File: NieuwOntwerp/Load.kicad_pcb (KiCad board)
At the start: 2 copper layers, 84 x 96 mm, 151 parts, among them J1 USB_C_Receptacle_USB2.0, J10 Conn_01x02, J2 Conn_01x02, J3 Conn_01x03, J4 Conn_01x02, J5 Conn_01x09_Male, J6 Conn_01x02, J7 Conn_01x03, J8 Conn_01x02, J9 Conn_01x02, Q1 Si2306, Q2 4809NG, Q3 IRF840, Q4 IRF840, Q5 IRF840, Q6 Si2306, T1 EE13, U1 ESP12E, U10 PC817, U11 TL431, U12 LM1117-3.3, U2 FT231XQ, U3 LM358, U4 MCP4725A0, U5 LM358, U6 INA219, U7 PCF8574, U8 SSD1306, U9 LNK364D

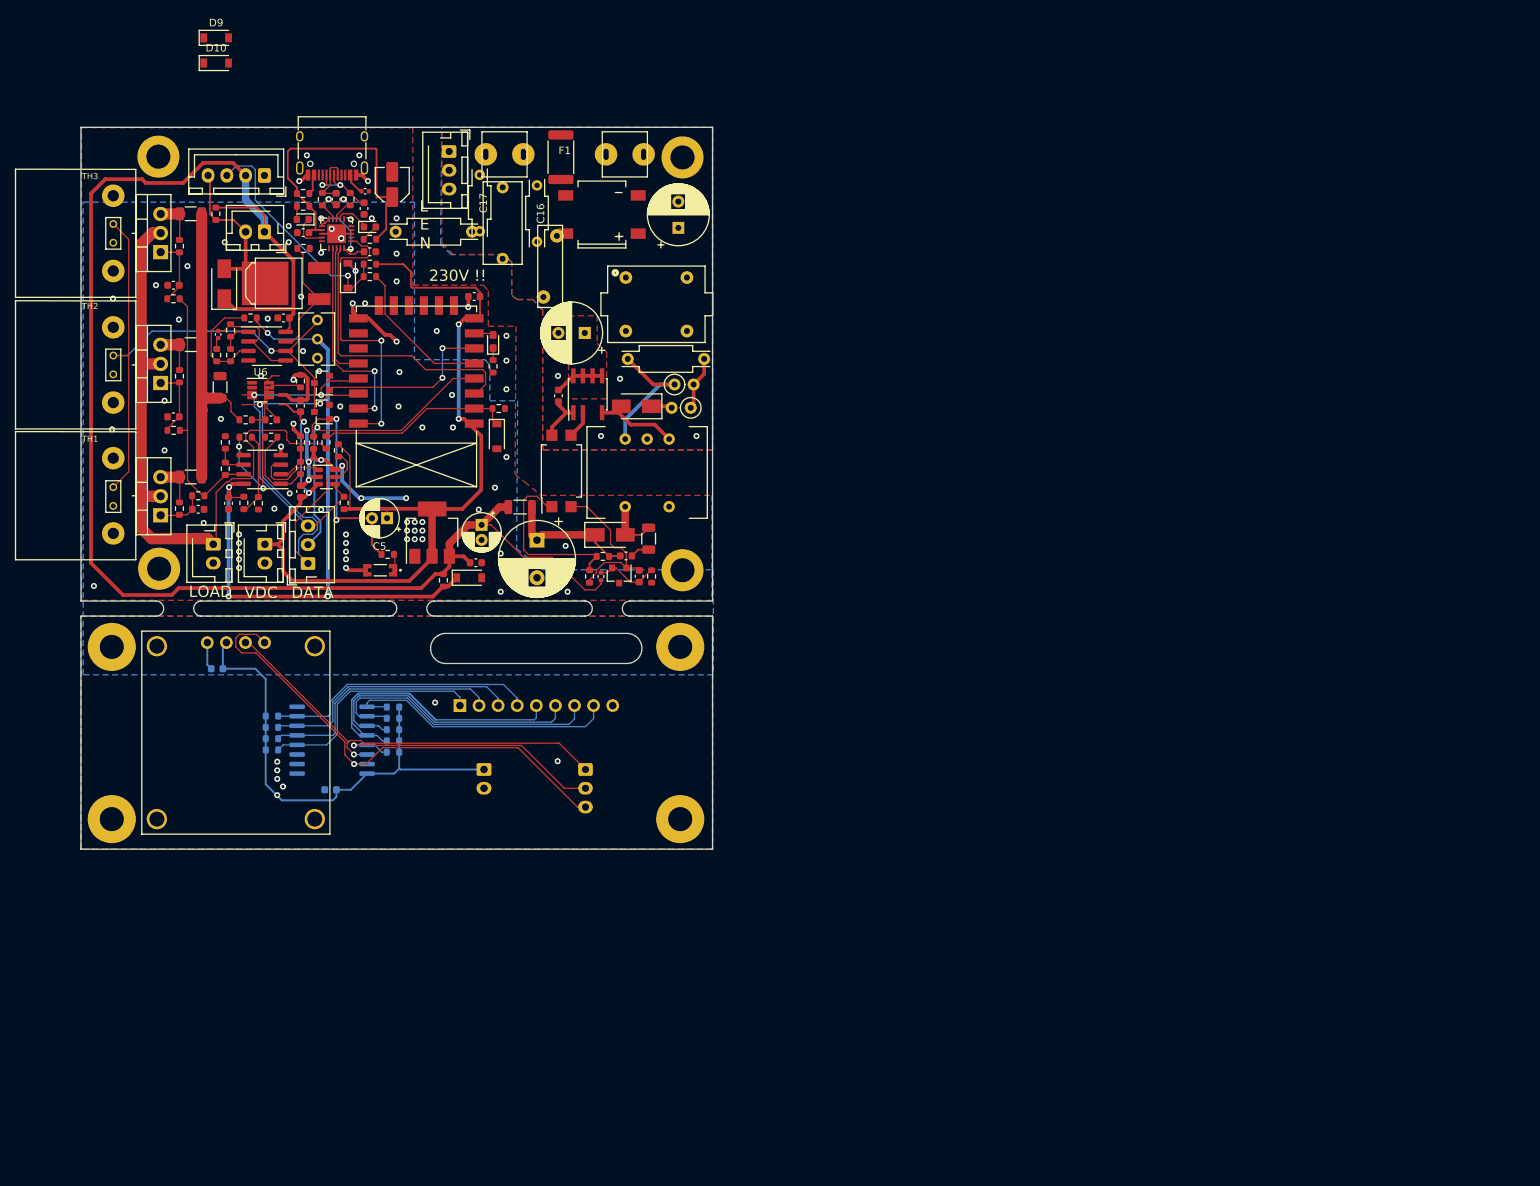
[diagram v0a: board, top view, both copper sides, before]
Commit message: Print_update
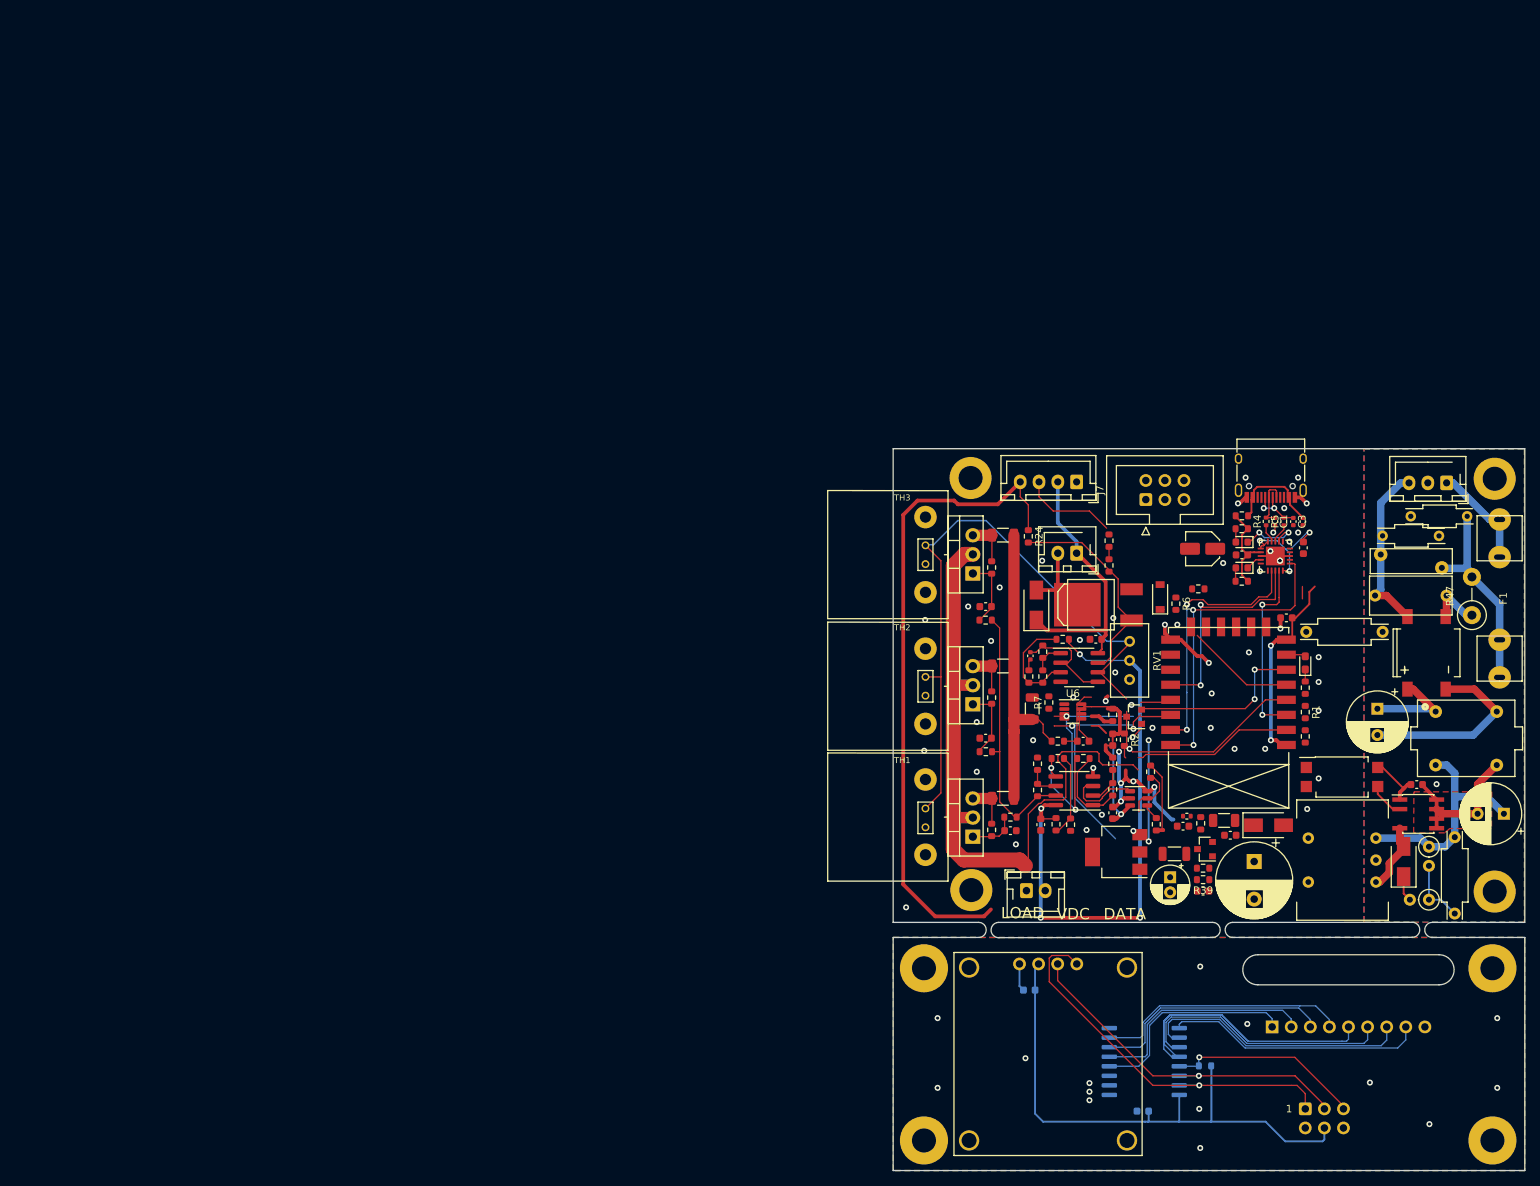
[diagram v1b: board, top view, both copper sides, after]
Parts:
- removed C5: 100uF, Capacitor_THT:CP_Radial_D5.0mm_P2.00mm
- removed D1: BZT52C-3V6, Diode_SMD:D_SOD-123
- removed D10, D9: MMSZ5225/3V, Diode_SMD:D_SOD-123
- removed D3: 1N4148, Diode2:DIO_LL4148
- removed D8: BZT52C-5V1, Diode_SMD:D_SOD-123
- removed J4, J8: Conn_01x02, Connector2:JST_XH_B2B-XH-AM_1x02_P2.50mm_Vertical
- removed Q1: Si2306, Package_TO_SOT_SMD:SOT-23
- removed R40, R41, R42, R45, R46, R55, R56: 10k, Resistor_SMD:R_0603_1608Metric
- removed R57: 1K2, Resistor_SMD:R_0603_1608Metric
- C1, C3: footprint Capacitor_SMD:C_0603_1608Metric -> Capacitor_SMD:C_0402_1005Metric
- C6: value 470pF -> 4,7nF
- J3, J7: value Conn_01x03 -> Din_02x03; footprint Connector2:JST_XH_B3B-XH-AM_1x03_P2.50mm_Vertical -> Connector_IDC:IDC-Header_2x03_P2.54mm_Vertical
- R1: value 330K -> 10K
- R2: value 10k -> 100K
- R20: value 100K -> 4K7
- R39: value 10k -> 0R; moved to F.Cu
- R4, R5: footprint Resistor_SMD:R_0603_1608Metric -> Resistor_SMD:R_0402_1005Metric
- R47: footprint Resistor_SMD:R_2512_6332Metric -> Resistor_THT:R_Axial_DIN0411_L9.9mm_D3.6mm_P5.08mm_Vertical
- R51: value 150 -> 1K2
- R54: value 6K8 -> 5K6
- R6: value 1K -> 10K
- R7: value 56K -> 27K
- RV1: footprint Potentiometer_THT:Potentiometer_Bourns_3266Y_Vertical -> Potentiometer_THT:Potentiometer_Bourns_3296W_Vertical
- U11: value TL431 -> TL432
- moved J9 139.8 mm to (190.4, 50.5), turned to 180 degrees
- moved C26 138.0 mm to (198.1, 94.6)
- moved F1 137.6 mm to (197.5, 65.9), turned to 90 degrees
- moved R47 135.6 mm to (193.8, 68.1)
- moved R1 135.1 mm to (171.6, 81.0), turned to 270 degrees
- moved R12 134.4 mm to (163.2, 63.6)
- moved D4 133.2 mm to (163.2, 61.8)
- moved R4 132.6 mm to (166.4, 55.7)
- moved C34 132.3 mm to (176.8, 70.4)
- moved C2 132.2 mm to (171.3, 55.7), turned to 270 degrees
- moved C1 132.0 mm to (167.6, 55.7)
- moved C21 132.0 mm to (163.2, 60.1)
- moved FB1 132.0 mm to (163.2, 54.9)
- moved J1 132.0 mm to (167.1, 47.3)
- moved U2 132.0 mm to (167.7, 60.3)
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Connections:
- C35 pad 2: +5V -> +12V
- C6 pad 1: Net-(C6-Pad1) -> GND
- H1 pad 1: GND -> Earth
- H2 pad 1: Net-(H2-Pad1) -> Earth
- J2 pad 4: Net-(D6-Pad2) -> Net-(J2-Pad4)
- J3 pad 1: /Front/SCL -> /Front/SDA
- J3 pad 3: /Front/SDA -> /Front/SCL
- J7 pad 1: SCL -> SDA
- J7 pad 2: ~INT -> Net-(J7-Pad2)
- J7 pad 3: SDA -> SCL
- Q3 pad 2: LOAD -> SHUNT
- Q4 pad 2: LOAD -> SHUNT
- Q5 pad 2: LOAD -> SHUNT
- R1 pad 1: LOAD -> RTS
- R1 pad 2: ADC -> +3V3
- R10 pad 2: +5V -> +12V
- R11 pad 1: Net-(C6-Pad1) -> GND
- R18 pad 2: +5V -> +12V
- R2 pad 1: ADC -> GND
- R2 pad 2: GND -> FAN_OVERRIDE
- R24 pad 1: Net-(D6-Pad2) -> Net-(J2-Pad4)
- R24 pad 2: +12V -> Net-(Q2-Pad1)
- R28 pad 1: SHUNT -> GND
- R31 pad 1: GND -> SHUNT
- R31 pad 2: SHUNT -> LOAD
- R32 pad 1: SHUNT -> GND
- R33 pad 2: SHUNT -> LOAD
- R34 pad 2: GND -> SHUNT
- R37 pad 1: SHUNT -> GND
- R38 pad 2: Net-(J3-Pad2) -> Net-(J3-Pad5)
- R39 pad 1: VDC -> Net-(C31-Pad2)
- R39 pad 2: Net-(J5-Pad1) -> Net-(R39-Pad2)
- R54 pad 1: Net-(C31-Pad2) -> Net-(R39-Pad2)
- R6 pad 1: Net-(D3-Pad1) -> GND
- R6 pad 2: Net-(C5-Pad2) -> Net-(R6-Pad2)
- R7 pad 2: Net-(C5-Pad2) -> THERM
- RV1 pad 2: +5V -> +12V
- U1 pad 10: Net-(U1-Pad10) -> Net-(R6-Pad2)
- U1 pad 2: ADC -> Net-(U1-Pad2)
- U1 pad 4: ~INT -> FAN_OVERRIDE
- U1 pad 6: FAN_OVERRIDE -> ~INT
- U5 pad 8: +5V -> +12V
- U7 pad 10: Net-(J5-Pad7) -> Net-(J5-Pad6)
- U7 pad 11: Net-(J5-Pad6) -> Net-(J5-Pad7)
- U7 pad 12: Net-(J5-Pad5) -> Net-(J5-Pad8)
- U7 pad 13: Net-(J3-Pad2) -> Net-(J3-Pad5)
- U7 pad 9: Net-(J5-Pad8) -> Net-(J5-Pad5)
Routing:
- net SHUNT: track 41.9 -> 186.8 mm
- net +5V: track 96.1 -> 0.00 mm, vias 4 -> 0
- net +12V: track 203.2 -> 113.9 mm, vias 0 -> 5
- net LOAD: track 88.2 -> 0.00 mm
- net Net-(J2-Pad4): track 0.00 -> 87.6 mm
- net +3V3: track 137.2 -> 54.3 mm, vias 4 -> 3
- net ~INT: track 40.2 -> 0.00 mm, vias 1 -> 0
- net Net-(J3-Pad2): track 38.0 -> 0.00 mm, vias 1 -> 0
- net VCC: track 40.8 -> 12.6 mm
- net Net-(C16-Pad2): track 0.00 -> 26.6 mm
- net Net-(J3-Pad5): track 0.00 -> 26.0 mm, vias 0 -> 1
- net ADC: track 26.0 -> 0.00 mm
- net Net-(C23-Pad2): track 0.00 -> 25.2 mm
- net Net-(R51-Pad1): track 23.5 -> 0.00 mm
- net FAN_OVERRIDE: track 23.2 -> 46.6 mm, vias 2 -> 3
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- removed copper zone on B.Cu, net GND
- removed copper zone on F.Cu, net GND
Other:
- outline, holes or cut-outs redrawn
- board text added: "1"
- board text added: "NC"
- board text removed: "230V !!"
- board text removed: "E"
- board text removed: "L"
- board text removed: "N"
